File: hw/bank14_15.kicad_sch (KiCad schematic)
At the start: 23 parts, among them U2 AT25SL641, U24 XC7A35T-FTG256

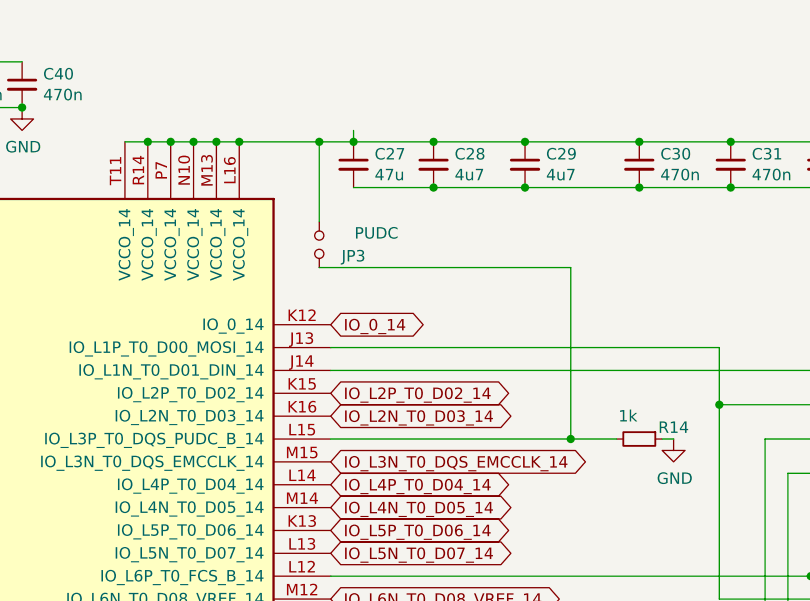
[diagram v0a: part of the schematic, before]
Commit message: layout finished (draft)
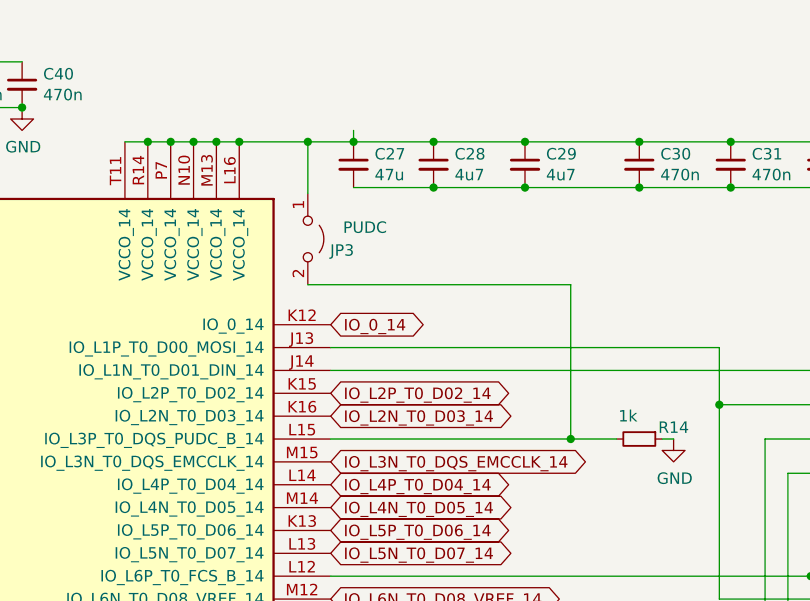
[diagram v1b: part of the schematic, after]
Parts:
- JP3: symbol Device:Jumper_NO_Small -> Jumper:Jumper_2_Open
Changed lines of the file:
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@@
   (junction (at 92.71 30.48) (diameter 0) (color 0 0 0 0)
   )
+  (junction (at 143.51 34.29) (diameter 0) (color 0 0 0 0)
+  )
   (junction (at 180.34 34.29) (diameter 0) (color 0 0 0 0)
   )
@@
   (junction (at 69.85 30.48) (diameter 0) (color 0 0 0 0)
   )
-  (junction (at 144.78 34.29) (diameter 0) (color 0 0 0 0)
-  )
   (junction (at 125.73 34.29) (diameter 0) (color 0 0 0 0)
   )
@@
     (stroke (width 0) (type default))
   )
+  (wire (pts (xy 143.51 34.29) (xy 143.51 40.005))
+    (stroke (width 0) (type default))
+  )
   (wire (pts (xy 190.5 39.37) (xy 200.66 39.37))
     (stroke (width 0) (type default))
@@
     (stroke (width 0) (type default))
   )
-  (wire (pts (xy 172.72 48.26) (xy 172.72 67.31))
+  (wire (pts (xy 172.72 50.165) (xy 172.72 67.31))
     (stroke (width 0) (type default))
   )
@@
     (stroke (width 0) (type default))
   )
-  (wire (pts (xy 144.78 48.26) (xy 172.72 48.26))
-    (stroke (width 0) (type default))
-  )
-  (wire (pts (xy 144.78 43.18) (xy 144.78 34.29))
+  (wire (pts (xy 143.51 50.165) (xy 172.72 50.165))
     (stroke (width 0) (type default))
   )
@@
     (stroke (width 0) (type default))
   )
-  (wire (pts (xy 135.89 34.29) (xy 144.78 34.29))
-    (stroke (width 0) (type default))
-  )
   (wire (pts (xy 203.2 78.74) (xy 253.365 78.74))
     (stroke (width 0) (type default))
@@
     (stroke (width 0) (type default))
   )
-  (wire (pts (xy 144.78 34.29) (xy 148.59 34.29))
+  (wire (pts (xy 135.89 34.29) (xy 143.51 34.29))
     (stroke (width 0) (type default))
   )
@@
   )
   (wire (pts (xy 200.66 71.12) (xy 196.85 71.12))
+    (stroke (width 0) (type default))
+  )
+  (wire (pts (xy 143.51 34.29) (xy 148.59 34.29))
     (stroke (width 0) (type default))
   )
@@
     )
   )
-  (symbol (lib_id "Device:Jumper_NO_Small") (at 144.78 45.72 270) (unit 1)
-    (in_bom yes) (on_board yes) (dnp no)
-    (property "Reference" "JP3" (at 148.59 46.99 90)
-      (effects (font (size 1.27 1.27)))
-    )
-    (property "Value" "PUDC" (at 151.13 44.45 90)
-      (effects (font (size 1.27 1.27)))
-    )
-    (property "Footprint" "Connector_PinHeader_2.54mm:PinHeader_1x02_P2.54mm_Vertical" (at 144.78 45.72 0)
-      (effects (font (size 1.27 1.27)) hide)
-    )
-    (property "Datasheet" "~" (at 144.78 45.72 0)
-      (effects (font (size 1.27 1.27)) hide)
-    )
+  (symbol (lib_id "Jumper:Jumper_2_Open") (at 143.51 45.085 270) (unit 1)
+    (in_bom yes) (on_board yes) (dnp no)
+    (property "Reference" "JP3" (at 147.32 46.355 90)
+      (effects (font (size 1.27 1.27)))
+    )
+    (property "Value" "PUDC" (at 149.86 43.815 90)
+      (effects (font (size 1.27 1.27)))
+    )
+    (property "Footprint" "Connector_PinHeader_2.54mm:PinHeader_1x02_P2.54mm_Vertical" (at 143.51 45.085 0)
+      (effects (font (size 1.27 1.27)) hide)
+    )
+    (property "Datasheet" "~" (at 143.51 45.085 0)
+      (effects (font (size 1.27 1.27)) hide)
+    )
